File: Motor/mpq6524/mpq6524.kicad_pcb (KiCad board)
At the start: 2 copper layers, 33.6 x 27 mm, 11 parts, among them J1 OQ0212500000G, J2 Conn_02x03_Odd_Even, U1 MPQ6524GRE-AEC1-P, U2 TPS5410DR

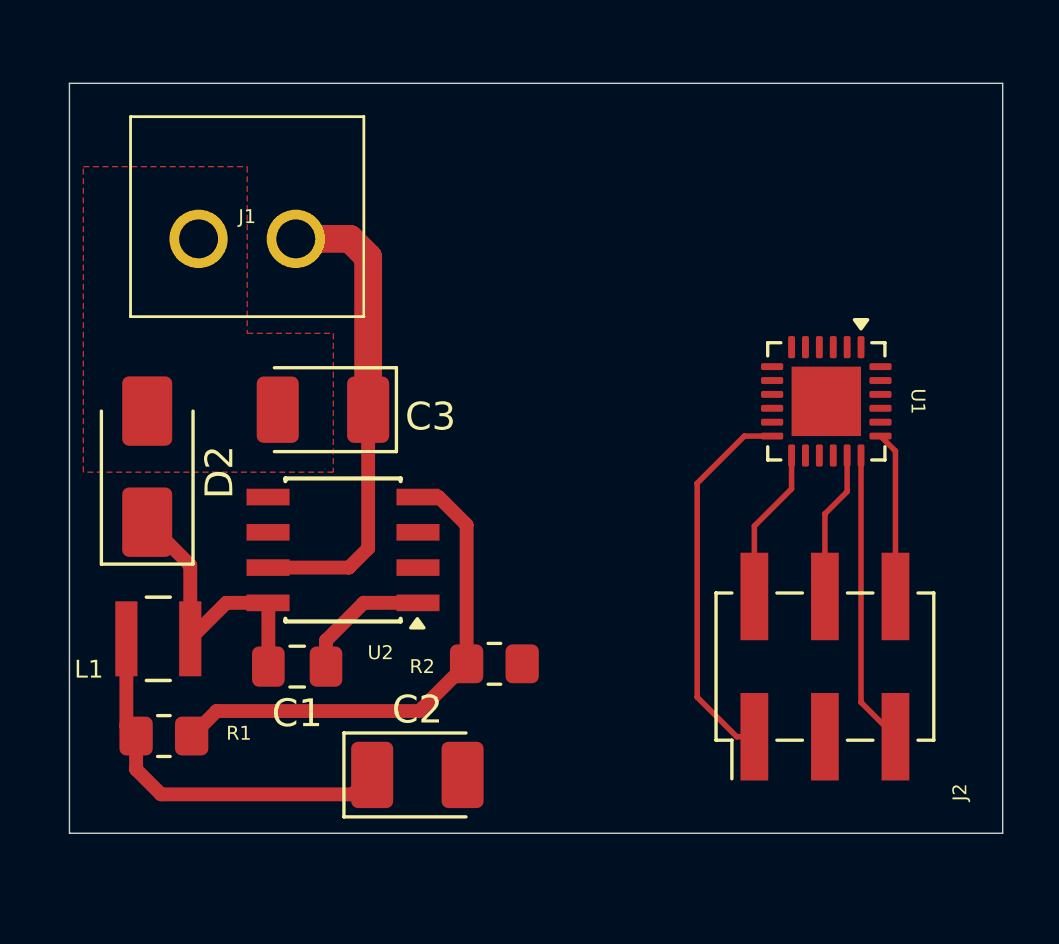
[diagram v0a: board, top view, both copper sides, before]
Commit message: Paths
Route some paths
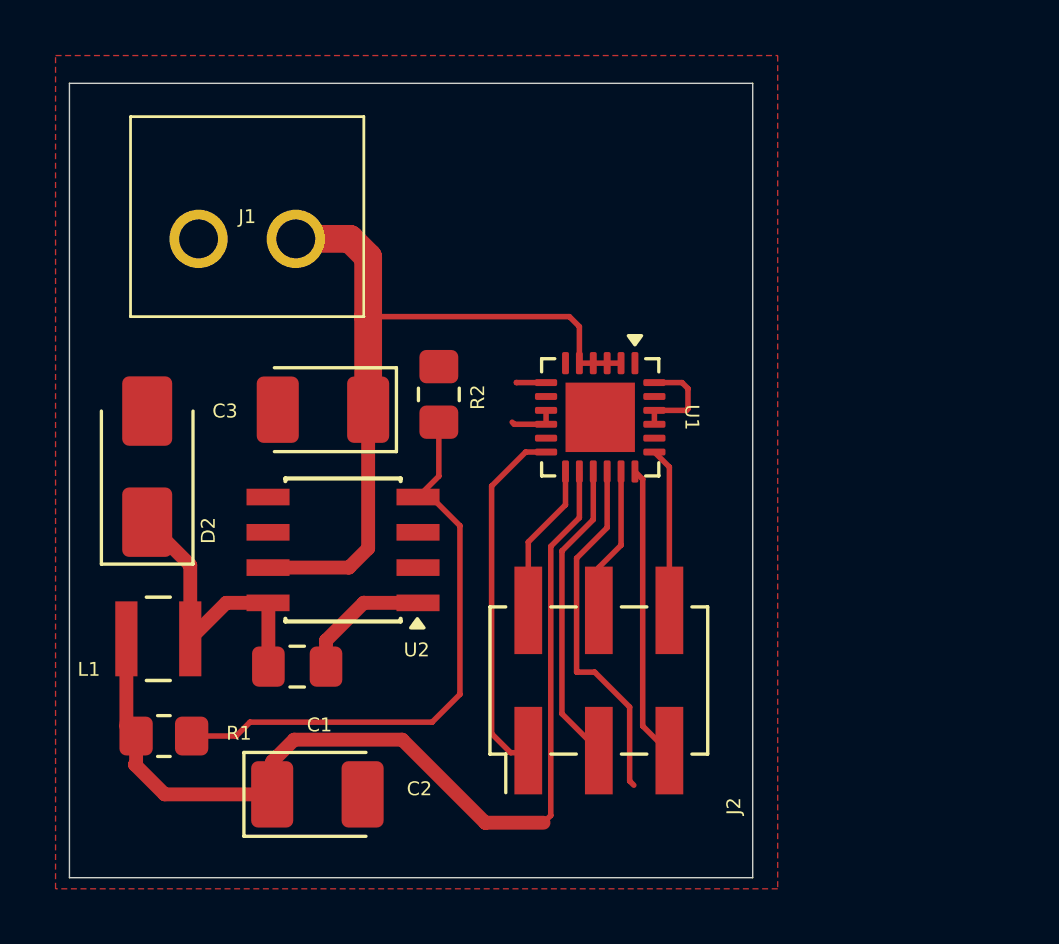
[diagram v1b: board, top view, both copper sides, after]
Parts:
- moved R2 9.90 mm to (161.8, 70.2), turned to 90 degrees
- moved U1 8.16 mm to (167.6, 71.0)
- moved J2 8.16 mm to (167.6, 80.5)
- moved C2 3.67 mm to (157.4, 84.6)
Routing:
- net +3V3: track 14.0 -> 35.8 mm
- net GND: track 0.00 -> 19.6 mm
- net /fault: track 0.00 -> 11.1 mm
- net +12V: track 17.3 -> 27.8 mm
- net Net-(U2-VSENSE): track 18.1 -> 21.3 mm
- net /MotorEnable: track 13.8 -> 13.0 mm
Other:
- board size 33.6 x 27 mm -> 24.6 x 28.6 mm
